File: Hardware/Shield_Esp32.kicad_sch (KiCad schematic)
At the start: 45 parts, among them J1 Conn_01x02_Male, J10 Conn_01x02_Male, J11 Conn_01x02_Male, J12 Conn_01x02_Male, J13 Conn_01x02_Male, J14 Conn_01x02_Male, J15 Conn_01x02_Male, J16 Conn_01x02_Male, J17 Conn_01x02_Male, J18 Conn_01x02_Male, J19 Conn_01x02_Male, J2 Conn_01x02_Male, J20 Conn_01x02_Male, J21 Conn_01x02_Male, J22 Conn_01x02_Male, J23 Conn_01x02_Male, J3 Conn_02x13_Odd_Even, J4 Conn_01x15, J5 Conn_01x15, J6 Conn_01x02_Male, J7 Conn_01x02_Male, J8 Conn_01x03_Male, J9 Conn_01x02_Male

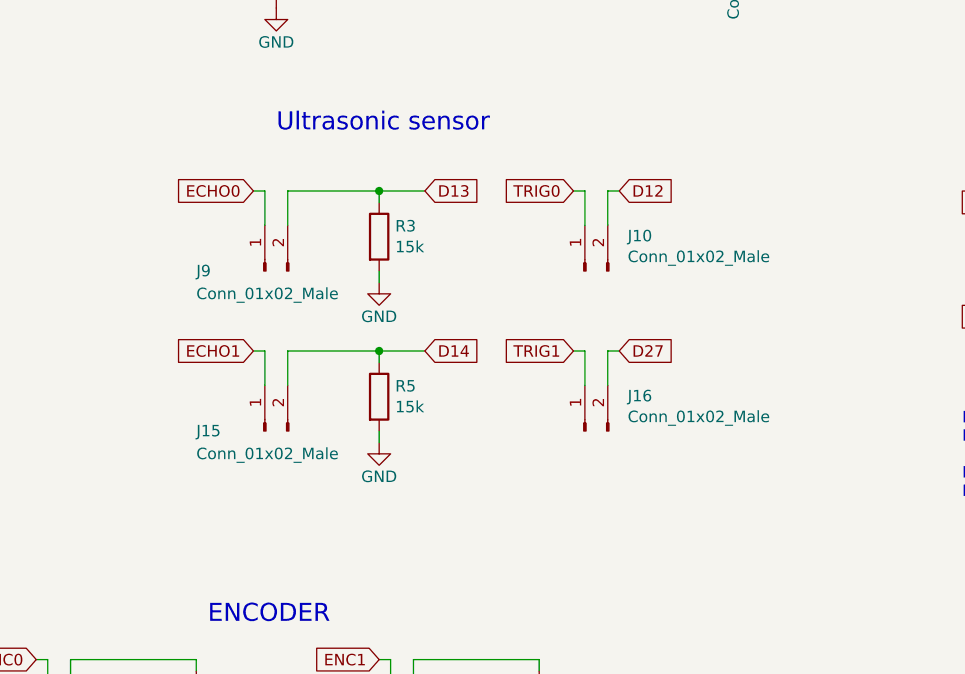
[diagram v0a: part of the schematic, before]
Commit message: update pcb
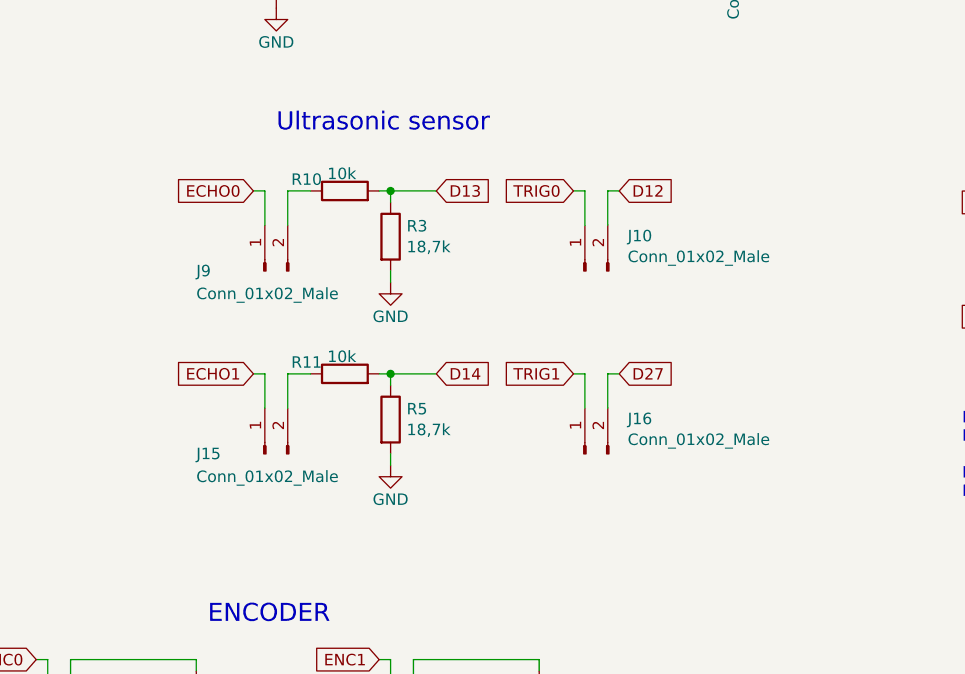
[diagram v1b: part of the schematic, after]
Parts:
- added R10, R11: 10k, Resistor_SMD:R_0805_2012Metric, symbol Device:R
- R3, R5: value 15k -> 18,7k
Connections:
- net D13: now also R10.2; no longer J9.2 (Pin_2)
- net D14: now also R11.2; no longer J15.2 (Pin_2)
- new net: J9.2 (Pin_2), R10.1
- new net: J15.2 (Pin_2), R11.1
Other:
- moved on the sheet: J15, J16, R3, R5
